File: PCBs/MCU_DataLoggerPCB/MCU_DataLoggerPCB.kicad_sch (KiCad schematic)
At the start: 25 parts, among them U1 24LC1025, U2 24LC1025, U3 DS1337S+, U4 ATMEGA328P-AU, Y1 32.768 kHz, Y2 16 MHz

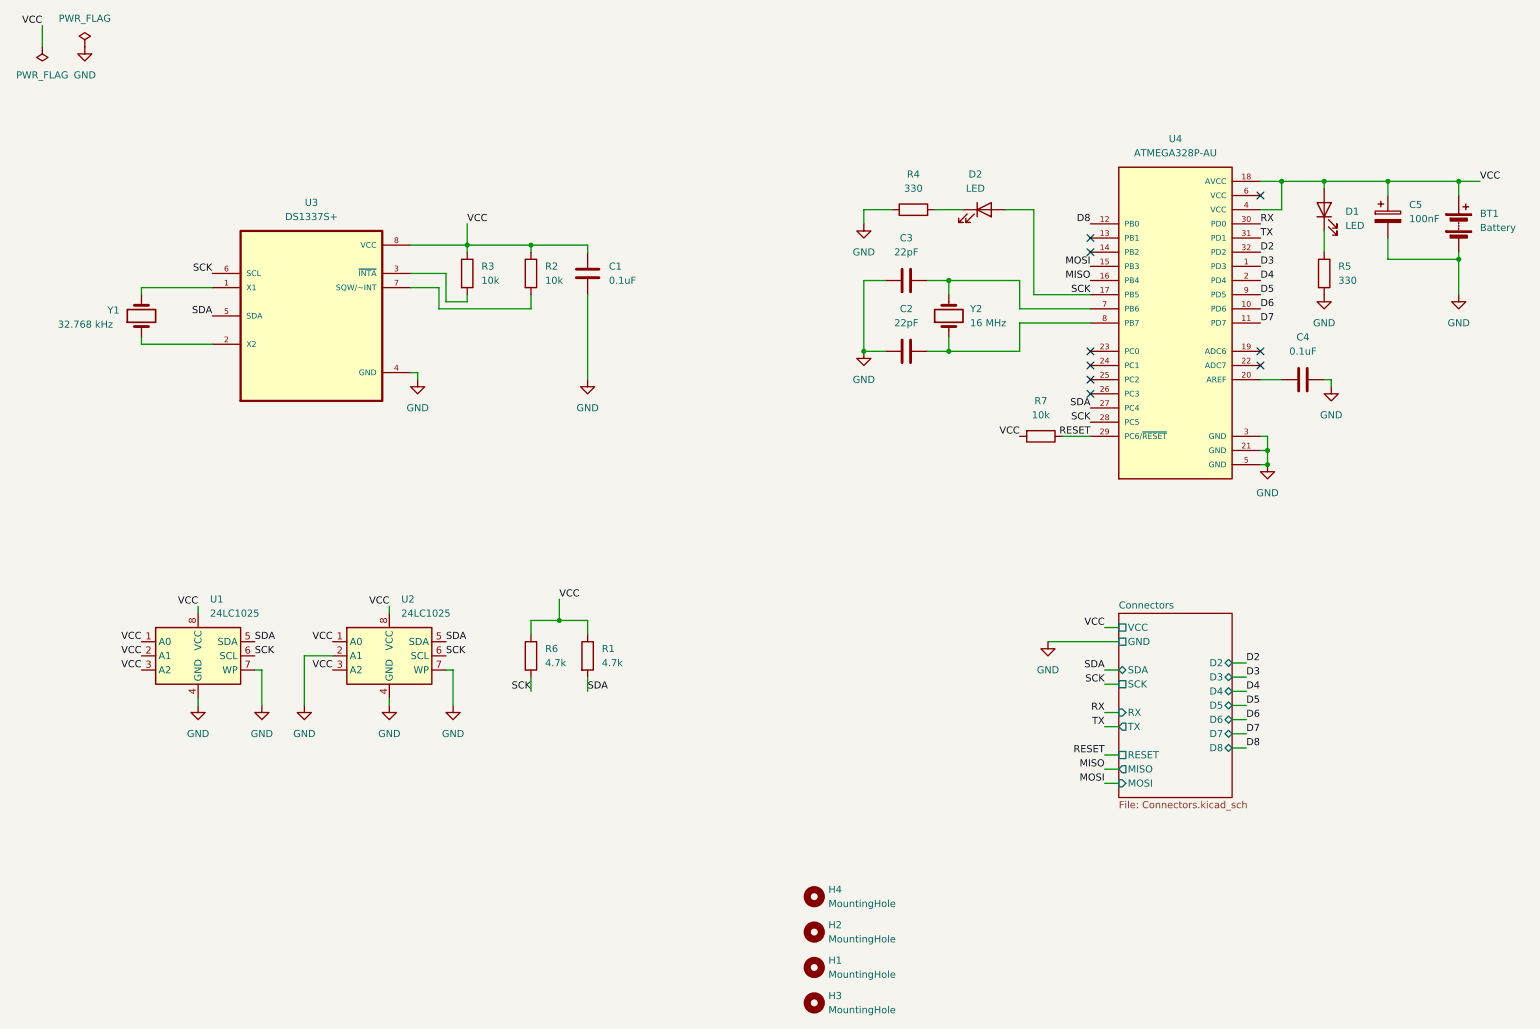
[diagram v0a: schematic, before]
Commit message: Project: completed comments
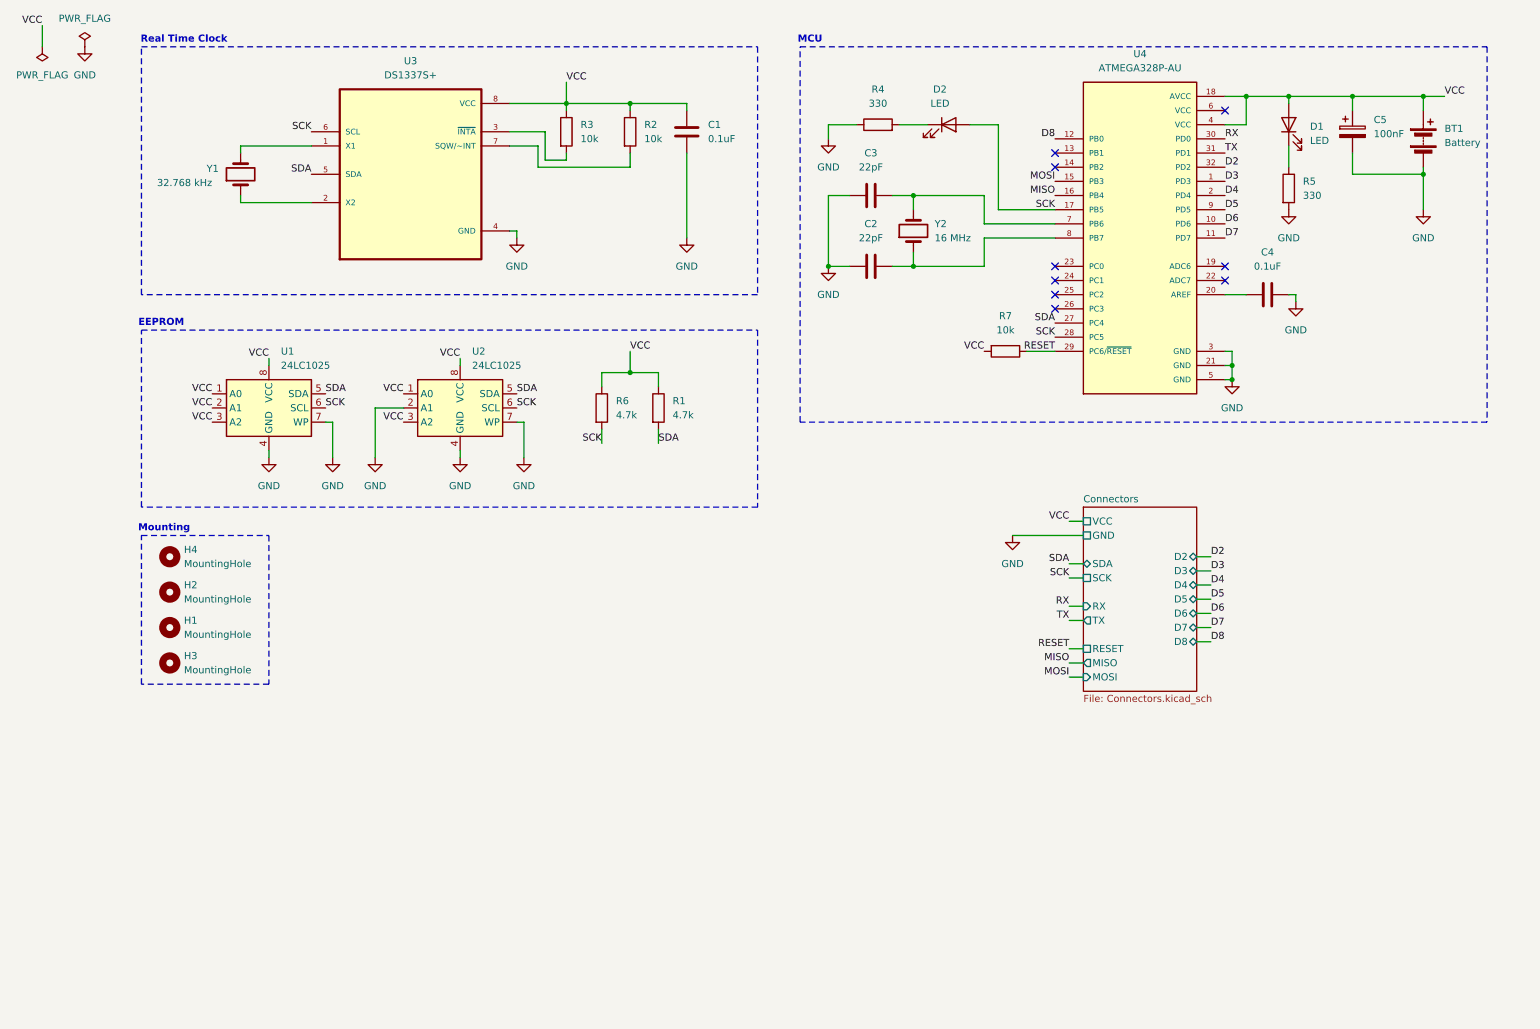
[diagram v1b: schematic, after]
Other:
- note added: "EEPROM"
- note added: "MCU"
- note added: "Mounting"
- note added: "Real Time Clock"
- moved on the sheet: BT1, C1, C2, C3, C4, C5, D1, D2, H1, H2, H3, H4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
